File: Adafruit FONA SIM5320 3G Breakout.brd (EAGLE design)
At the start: 45.7 x 49.5 mm, 46 parts, among them CN2 JSTPH, SW1 KMR2, U1 SIM5320, U2 MCP73831T-2ACI/OT, X1 uFL, X2 MicroB, X3 uFL, X6 SIM_LOCKAMPHENOL

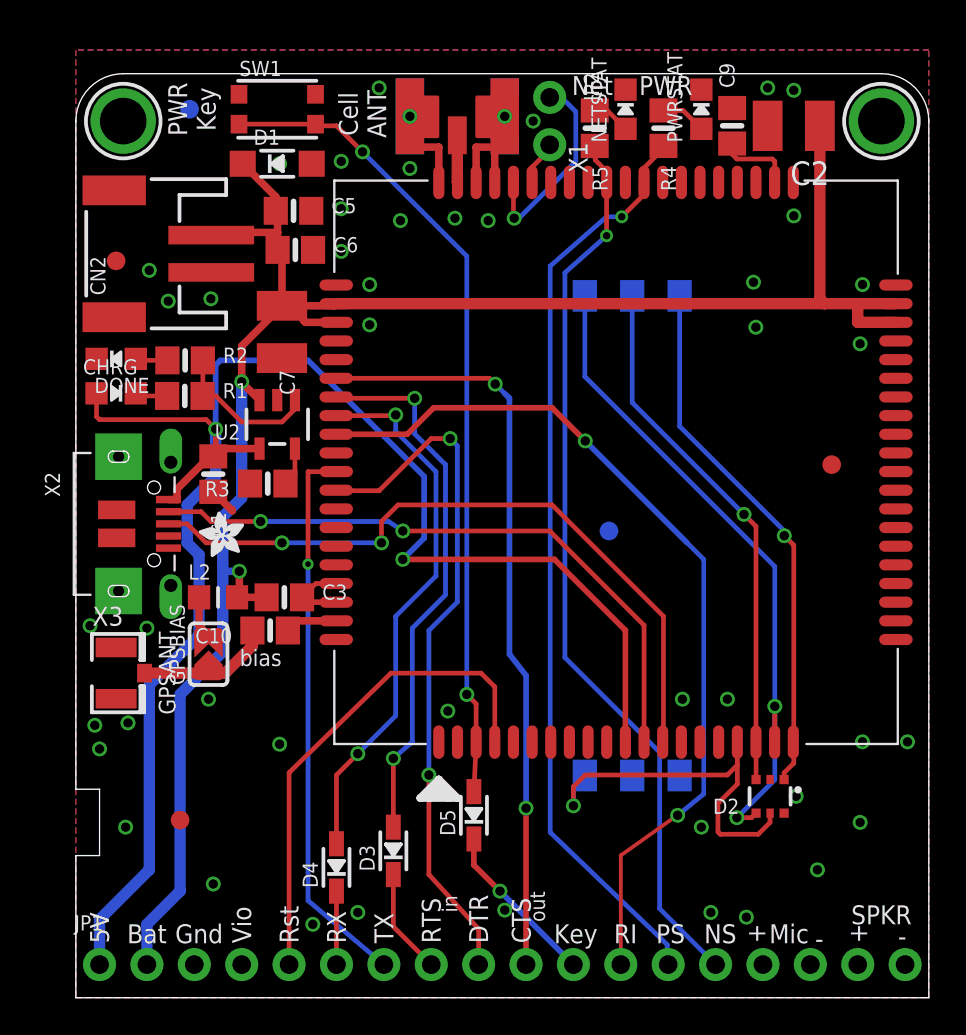
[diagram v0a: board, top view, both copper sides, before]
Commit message: 部品をPCB Fusion化
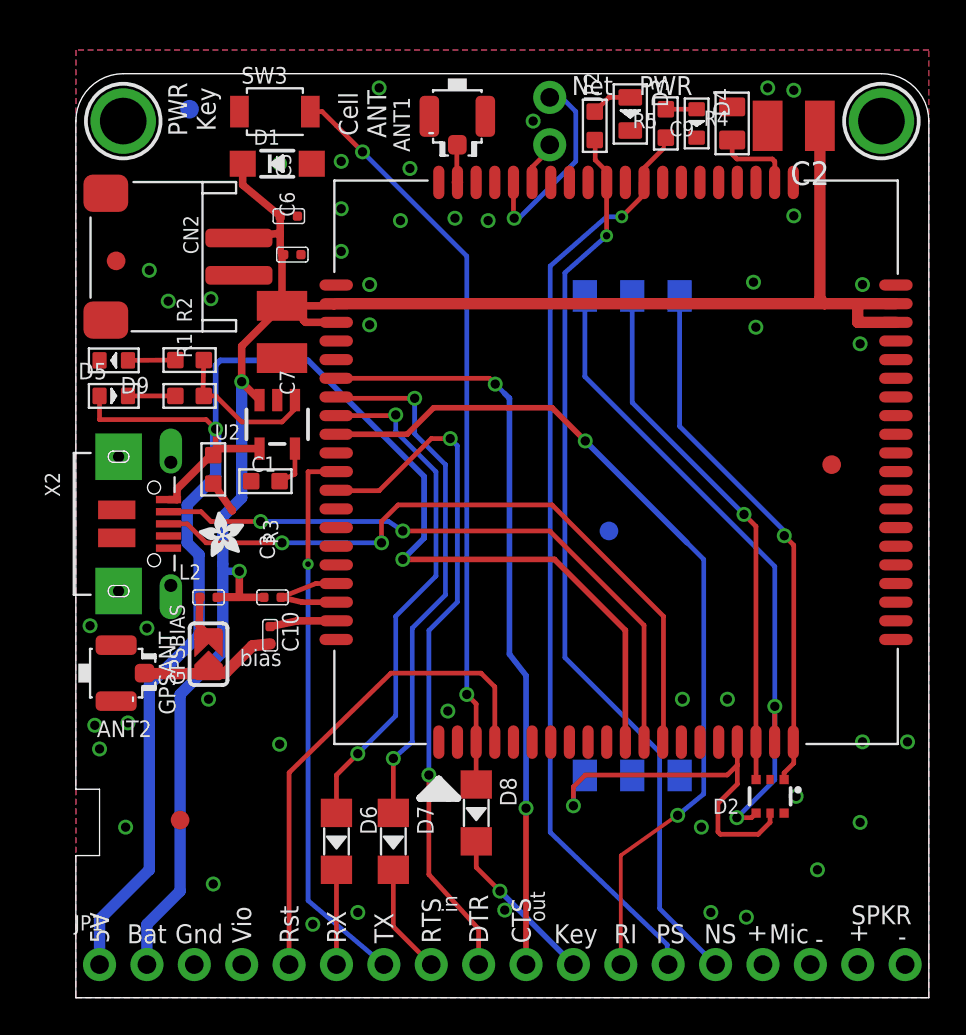
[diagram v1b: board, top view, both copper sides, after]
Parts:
- removed CHRG: ORANGE, microbuilder:CHIPLED_0805_NOOUTLINE
- removed DONE, PWRSTAT: GREEN, microbuilder:CHIPLED_0805_NOOUTLINE
- removed NETSTAT: RED, microbuilder:CHIPLED_0805_NOOUTLINE
- removed SW1: KMR2, microbuilder:BTN_KMR2_4.6X2.8
- removed X1: uFL, microbuilder:SMA_EDGELAUNCH_UFL
- removed X3: uFL, microbuilder:U.FL
- added ANT1, ANT2: U-FL, Seeed-Connector:U-FL3P-SMD-2.6X2.6X1.0MM
- added D6, D7, D8: 1N4148, Seeed-Diode:LL-34
- added D9: GREEN-0603, Seeed-LED:LED-0603
- added SW3: B3U-1000P-2P-SMD, Seeed-Switch:SW2-2.6-3.0X2.5X1.2+0.4MM
- C1: value 10µF -> 10uf; device microbuilder:0805-NO -> Seeed-Capacitor:C0603
- C10, C3, C6: value 33pF -> 33pf; device microbuilder:0805-NO -> Seeed-Capacitor:C0402
- C5: value 10pF -> 10pf; device microbuilder:0805-NO -> Seeed-Capacitor:C0402
- C9: value 10uF -> 10uf; device microbuilder:0805-NO -> Seeed-Capacitor:C0805
- CN2: value JSTPH -> 2P-2.0-90D-SMD; device microbuilder:JSTPH2 -> Seeed-Connector:HW2-SMD-2.0-90D
- D3: value 1N4148 -> RED-0805; device microbuilder:SOD-323 -> Seeed-LED:LED-0805
- D4: value 1N4148 -> GREEN-0603; device microbuilder:SOD-323 -> Seeed-LED:LED-0603
- D5: value 1N4148 -> YELLOW-0603; device microbuilder:SOD-323 -> Seeed-LED:LED-0603
- L2: value 33nH -> 15NH-300MA; device microbuilder:_0805MP -> Seeed-Inductor:L0402
- R1: value 470 -> 470R; device microbuilder:0805-NO -> Seeed-Resistor:R0603
- R2, R3, R4, R5: device microbuilder:0805-NO -> Seeed-Resistor:R0603
- moved D4 44.3 mm to (33.3, 46.9), turned to 270 degrees
- moved D3 41.5 mm to (29.7, 47.4), turned to 270 degrees
- moved D5 29.6 mm to (2.03, 32.3), turned to 0 degrees
- moved C3 0.63 mm to (10.5, 21.5), turned to 90 degrees
- moved L2 0.51 mm to (7.11, 21.5)
- moved C5 0.38 mm to (11.4, 41.9), turned to 90 degrees
- moved C6 0.30 mm to (11.6, 39.8), turned to 90 degrees
- moved R4 0.28 mm to (31.6, 46.9), turned to 0 degrees
- moved CN2 0.28 mm to (3.79, 39.7), turned to 270 degrees
- moved C1 0.25 mm to (7.37, 28.3), turned to 0 degrees
- moved R1 0.25 mm to (6.10, 32.3), turned to 90 degrees
- moved C10 0.25 mm to (10.4, 19.4), turned to 0 degrees
- moved R2 0.24 mm to (6.10, 34.2), turned to 90 degrees
- moved R3 0.18 mm to (10.2, 27.7), turned to 270 degrees
- moved C9 0.13 mm to (35.2, 46.9), turned to 180 degrees
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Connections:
- net +5V: now also D5.+; no longer CHRG.A
- net CTS_5V: now also D7.C; no longer D3.C
- net GND: now also ANT1.GND1, ANT1.GND2, ANT2.GND1, ANT2.GND2, CN2.-, D3.-, D4.-, D9.-, SW3.1; no longer CN2.1, DONE.C, NETSTAT.C, PWRSTAT.C, SW1.A, SW1.A', X1.GND@1, X1.GND@2, X1.GND@3, X1.GND@4, X3.1, X3.2
- net GSM_ANT: now also ANT1.D; no longer X1.P
- net N$1: now also D5.-; no longer CHRG.C
- net N$3: now also ANT2.D; no longer X3.3
- net N$4: now also D4.+; no longer PWRSTAT.A
- net N$6: now also D9.+; no longer DONE.A
- net N$9: now also D3.+; no longer NETSTAT.A
- net PWRKEY: now also D8.A, SW3.2; no longer D5.A, SW1.B, SW1.B'
- net PWRKEY_5V: now also D8.C; no longer D5.C
- net RXD_5V: now also D6.C; no longer D4.C
- net UART_CTS: now also D7.A; no longer D3.A
- net UART_RXD: now also D6.A; no longer D4.A
- net VBAT: now also CN2.+; no longer CN2.2
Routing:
- net GND: track 17.8 -> 7.91 mm, vias 47 -> 45
- net PWRKEY: track 44.1 -> 40.1 mm
- net UART_RXD: track 29.3 -> 27.6 mm
- net RXD_5V: track 3.94 -> 5.08 mm
- net N$6: track 1.73 -> 2.54 mm
- net VBAT: track 104.7 -> 105.5 mm
- net N$4: track 2.44 -> 1.65 mm
- net N$7: track 2.81 -> 3.57 mm
- net UART_CTS: track 29.1 -> 28.3 mm
- net N$1: track 2.02 -> 2.54 mm
